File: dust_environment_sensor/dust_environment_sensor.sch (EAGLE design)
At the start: 36 parts, among them J1 3.6V Lithium C cell, U1 LTP5901, U2 LIS3DH, U3 SI7005, U4 TSL2560, U5 ATMEGA328P, X1 32.768KHz

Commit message: Latest Powerstrip changes
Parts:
- removed C31, C32: 22p, SparkFun:CAP0603
- removed C33, C34, C41: .1u, SparkFun:CAP0603
- removed JP2: AVR_SPI_PRG_6NS, SparkFun:AVR_SPI_PRG_6NS
- removed JP3: .1" header, con-lstb:MA06-2
- removed LED1: RED, led:LEDCHIPLED_0805
- removed R46: 10k, SparkFun:RESISTOR0603
- removed X1: 32.768KHz, WSNlib:XTALABS07
- added C10, C13, C15, C8, C9: 100n, rcl:C-EUC0603
- added C11, C12: TODO, rcl:C-EUC0603
- added C14: 10u, rcl:C-USC0603
- added IC2: ATMEGA644A, atmel:ATMEGA644A
- added J2: EXP, SparkFun-Connectors:AVR_SPI_PRG_6PTH
- added J3: XBEE_1-10SMT, Cool_Electricity:XBEE_1-10SMT
- added J4: XBEE_11-20SMT, Cool_Electricity:XBEE_11-20SMT
- added JP8: (no value), custom:FTDI_CABLESIP
- added JP9: JTAG, SparkFun-Connectors:M05X2PTH
- added LED2, LED3: (no value), led:LEDCHIPLED_0805
- added R5: 0R, resistor:R-US_R0603
- added U6: L3GD20, Cool_Electricity:L3GD20
- added X2: 32.768KHz, WSNlib:XTALABS07
- C1, C5, C6: device rcl:C-USC0603 -> rcl:C-EUC0603
- R4: value 120 -> 10k; device SparkFun:RESISTOR0603 -> resistor:R-US_R0603
- U5: value ATMEGA328P -> AMN41121; device SparkFun:ATMEGA168 -> Cool_Electricity:AMN41121
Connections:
- removed net ATMEGA_RX: JP3.7, U5.PD0(RXD)
- removed net ATMEGA_TX: JP3.9, U5.PD1(TXD)
- removed net MISO: JP2.1, U5.PB4(MISO)
- removed net MOSI: JP2.4, U5.PB3(MOSI/OC2)
- removed net N$4: C32.1, U5.PB7(XTAL2/TOSC2), X1.A
- removed net N$5: LED1.A, R4.1
- removed net SCLK: JP2.3, U5.PB5(SCK)
- new net ATMEGA_TO_FTDI: IC2.(PCINT25/TXD0)PD1, JP8.RXD
- new net EXP_CSN: IC2.(PCINT12/OC0B/!SS!)PB4, J2.5
- new net EXP_MISO: IC2.(PCINT14/MISO)PB6, J2.1
- new net EXP_MOSI: IC2.(PCINT13/MOSI)PB5, J2.4
- new net EXP_SCK: IC2.(PCINT15/SCK)PB7, J2.3
- new net FTDI_TO_ATMEGA: IC2.(PCINT24/RXD0)PD0, JP8.TXD
- new net GYRO_INT2: IC2.(PCINT11/OC0A/AIN1)PB3, U6.DRDY/INT2
- new net LED2: IC2.(PCINT28/OC1B)PD4, LED3.A
- new net N$6: C11.1, IC2.(PCINT22/TOSC1)PC6, X2.B
- new net N$7: C12.1, IC2.(PCINT23/TOSC2)PC7, X2.A
- new net PIR_OUT: IC2.(PCINT31/OC2A)PD7, U5.OUT
- new net PIR_VCC: IC2.(PCINT7/ADC7)PA7, U5.VDD
- new net TCK: IC2.(PCINT18/TCK)PC2, JP9.1
- new net TDI: IC2.(PCINT21/TDI)PC5, JP9.9
- new net TDO: IC2.(PCINT20/TDO)PC4, JP9.3
- new net TMS: IC2.(PCINT19/TMS)PC3, JP9.5
- net ACCEL_INT1: now also IC2.(PCINT0/ADC0)PA0; no longer U5.PD2(INT0)
- net ACCEL_INT2: now also IC2.(PCINT1/ADC1)PA1; no longer U5.PC0(ADC0)
- net GND: now also C11.2, C12.2, C13.2, C14.2, C15.2, C8.1, C9.1, IC2.GND, IC2.GND@1, IC2.GND@2, IC2.GND@3, J2.6, J3.GND, JP8.CTS, JP8.GND, JP9.10, JP9.2, LED2.C, LED3.C, U5.GND, U6.GND, U6.RES/GND@1, U6.RES/GND@2, U6.RES/GND@3, U6.RES/GND@4, U6.RES/GND@5; no longer C31.2, C32.2, C33.1, C34.1, JP2.6, JP3.1, JP3.3, LED1.C, U5.ADC6, U5.ADC7, U5.AGND, U5.GND@1, U5.GND@2
- net HUMID_VCC: now also IC2.(PCINT2/ADC2)PA2; no longer U5.PC2(ADC2)
- net I2C_SCL: now also IC2.(PCINT16/SCL)PC0, U6.SCL/SPC; no longer U5.PC5(ADC5/SCL)
- net I2C_SDA: now also IC2.(PCINT17/SDA)PC1, U6.SDA/SDI/SDO; no longer U5.PC4(ADC4/SDA)
- net LED1: now also IC2.(PCINT29/OC1A)PD5, LED2.A; no longer R4.2, U5.PC3(ADC3)
- net LIGHT_INT: now also IC2.(PCINT6/ADC6)PA6; no longer U5.PC1(ADC1)
- net MOTE_API_RX: now also IC2.(PCINT27/INT1)PD3, J3.DIN/!CONFIG; no longer JP3.10
- net MOTE_API_TX: now also IC2.(PCINT26/INT0)PD2, J3.DOUT; no longer JP3.8
- net MOTE_RADIO_INHIBIT: now also IC2.(PCINT5/ADC5)PA5; no longer U5.PB0(ICP)
- net MOTE_RESETN: now also J3.!RESET; no longer U5.PD7(AIN1)
- net MOTE_RX_CTSN: now also IC2.(PCINT8/XCK0/T0)PB0; no longer U5.PD6(AIN0)
- net MOTE_RX_RTSN: now also IC2.(PCINT30/OC2B/ICP)PD6, J4.!RTS!/AD6/DIO6; no longer U5.PD5(T1)
- net MOTE_SLEEPN: now also IC2.(PCINT4/ADC4)PA4, J3.!DTR!/SLEEP_RQ/DIO8; no longer U5.PB1(OC1A)
- net MOTE_TIMEN: now also IC2.(PCINT3/ADC3)PA3; no longer U5.PB2(SS/OC1B)
- net MOTE_TX_CTSN: now also IC2.(PCINT9/CLKO/T1)PB1; no longer U5.PD4(XCK/T0)
- net MOTE_TX_RTSN: now also IC2.(PCINT10/INT2/AIN0)PB2; no longer U5.PD3(INT1)
- net N$2: now also C15.1, U6.CAP; no longer C31.1, U5.PB6(XTAL1/TOSC1), X1.B
- net RST: now also C10.1, IC2.RESET, JP9.6, R4.1; no longer C41.1, JP2.5, R46.1, U5.PC6(/RESET)
- net RTS#: now also C10.2, JP8.RTS; no longer C41.2, JP3.11
- net VBATT: now also R5.2; no longer JP3.4
- net VCC: now also C13.1, C14.1, C8.2, C9.2, IC2.AVCC, IC2.VCC, IC2.VCC@1, IC2.VCC@2, J2.2, J3.VCC, JP9.4, R4.2, R5.1, U6.CS, U6.RES/VDD, U6.SDO/SA0, U6.VDD, U6.VDD_IO; no longer C33.2, C34.2, JP2.2, JP3.6, R46.2, U5.AVCC, U5.VCC@1, U5.VCC@2
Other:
- note added: "RX1"
- note added: "TX1"
- note removed: "AN0"
- note removed: "AN1"
- note removed: "AN2"
- note removed: "AN3"
- note removed: "AN4"
- note removed: "AN5"
- note removed: "DIG0"
- note removed: "DIG1"
- note removed: "DIG10 (PWM)"
- note removed: "DIG11 (PWM)"
- note removed: "DIG12"
- note removed: "DIG13"
- note removed: "DIG14"
- note removed: "DIG15"
- note removed: "DIG16"
- note removed: "DIG17"
- note removed: "DIG18"
- note removed: "DIG19"
- note removed: "DIG2"
- note removed: "DIG3"
- note removed: "DIG4"
- note removed: "DIG5 (PWM)"
- note removed: "DIG6 (PWM)"
- note removed: "DIG7"
- note removed: "DIG8"
- note removed: "DIG9 (PWM)"
- moved on the sheet: C4, J1, R4

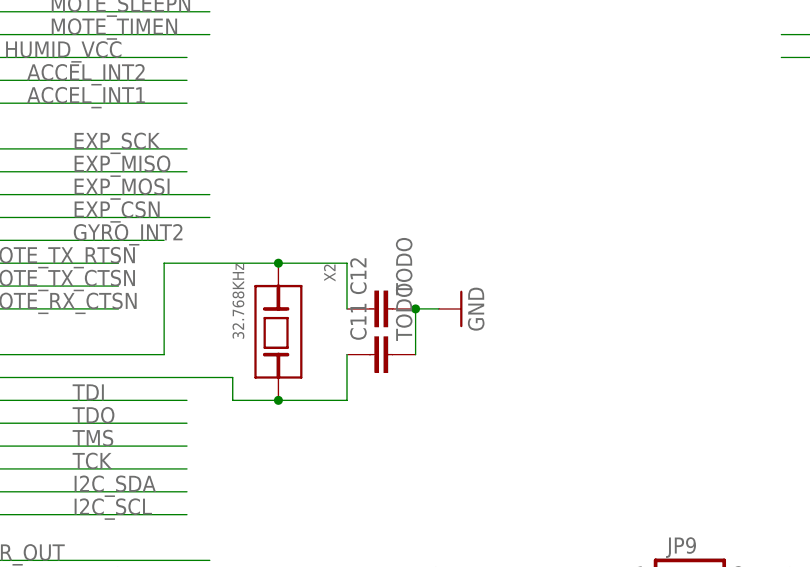
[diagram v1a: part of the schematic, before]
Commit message: BOM Updates
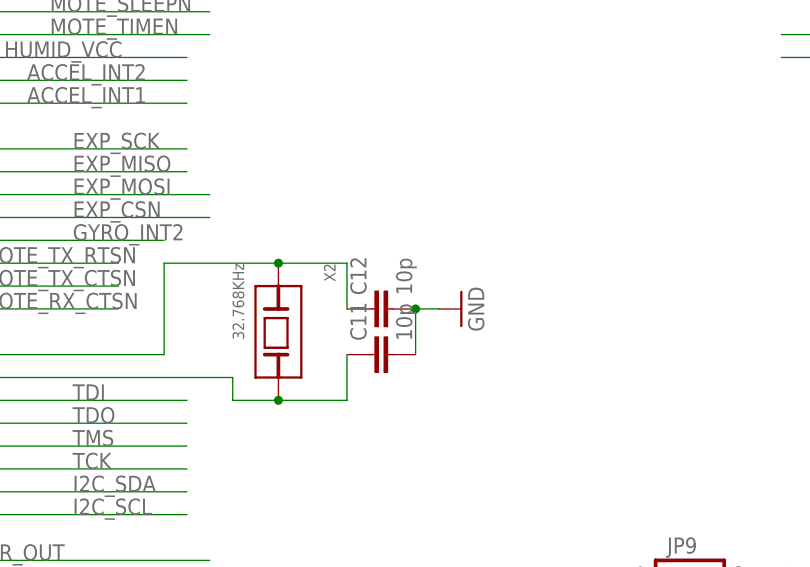
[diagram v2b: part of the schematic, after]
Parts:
- C11, C12: value TODO -> 10p
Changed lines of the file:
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@@
 <part name="GND24" library="SparkFun" deviceset="GND" device=""/>
 <part name="P+3" library="supply1" deviceset="VCC" device=""/>
-<part name="C11" library="rcl" deviceset="C-EU" device="C0603" value="TODO"/>
-<part name="C12" library="rcl" deviceset="C-EU" device="C0603" value="TODO"/>
+<part name="C11" library="rcl" deviceset="C-EU" device="C0603" value="10p"/>
+<part name="C12" library="rcl" deviceset="C-EU" device="C0603" value="10p"/>
 <part name="GND19" library="SparkFun" deviceset="GND" device=""/>
 <part name="X2" library="WSNlib" deviceset="XTAL" device="ABS07" value="32.768KHz"/>
